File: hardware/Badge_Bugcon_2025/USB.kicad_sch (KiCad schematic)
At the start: 37 parts, among them J10 Battery, J3 USB_A, J4 USB_A, J6 USB_A, P4 USB_C_Plug_USB2.0, Q1 DMG3415U-7, SW1 ON, SW4 On, U1 USB3740B-AI9, U3 SL2.1A, U5 MCP73831T-2ATI/OT, Y5 12MHz

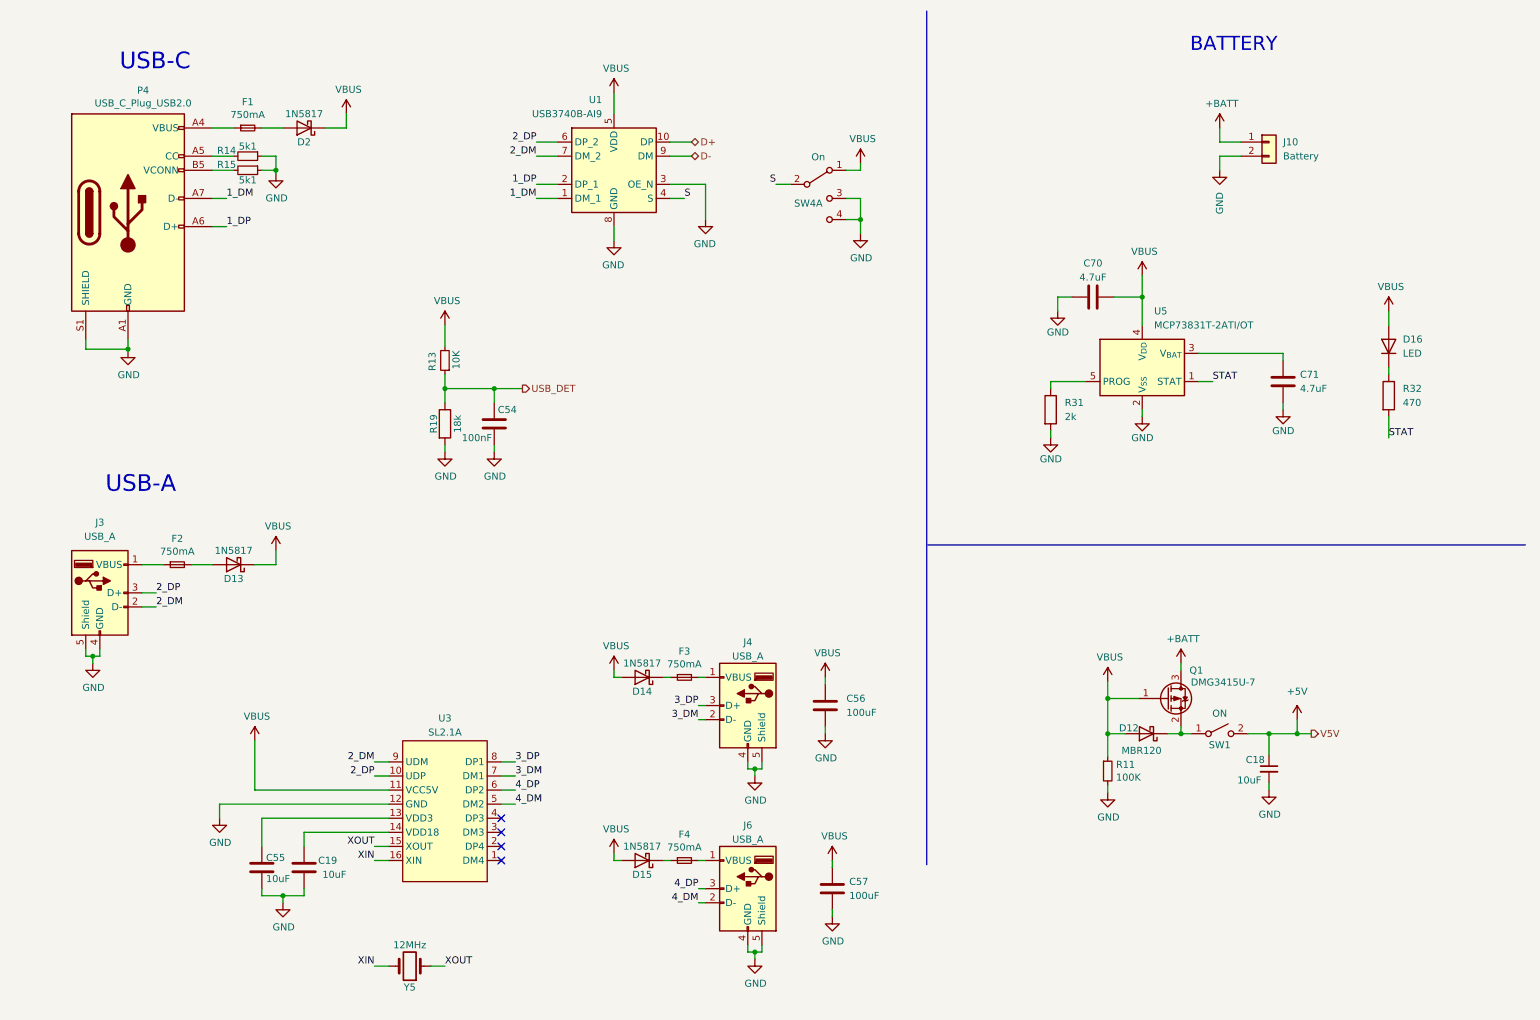
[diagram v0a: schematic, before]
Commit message: feat(Hw):Update_Schematic
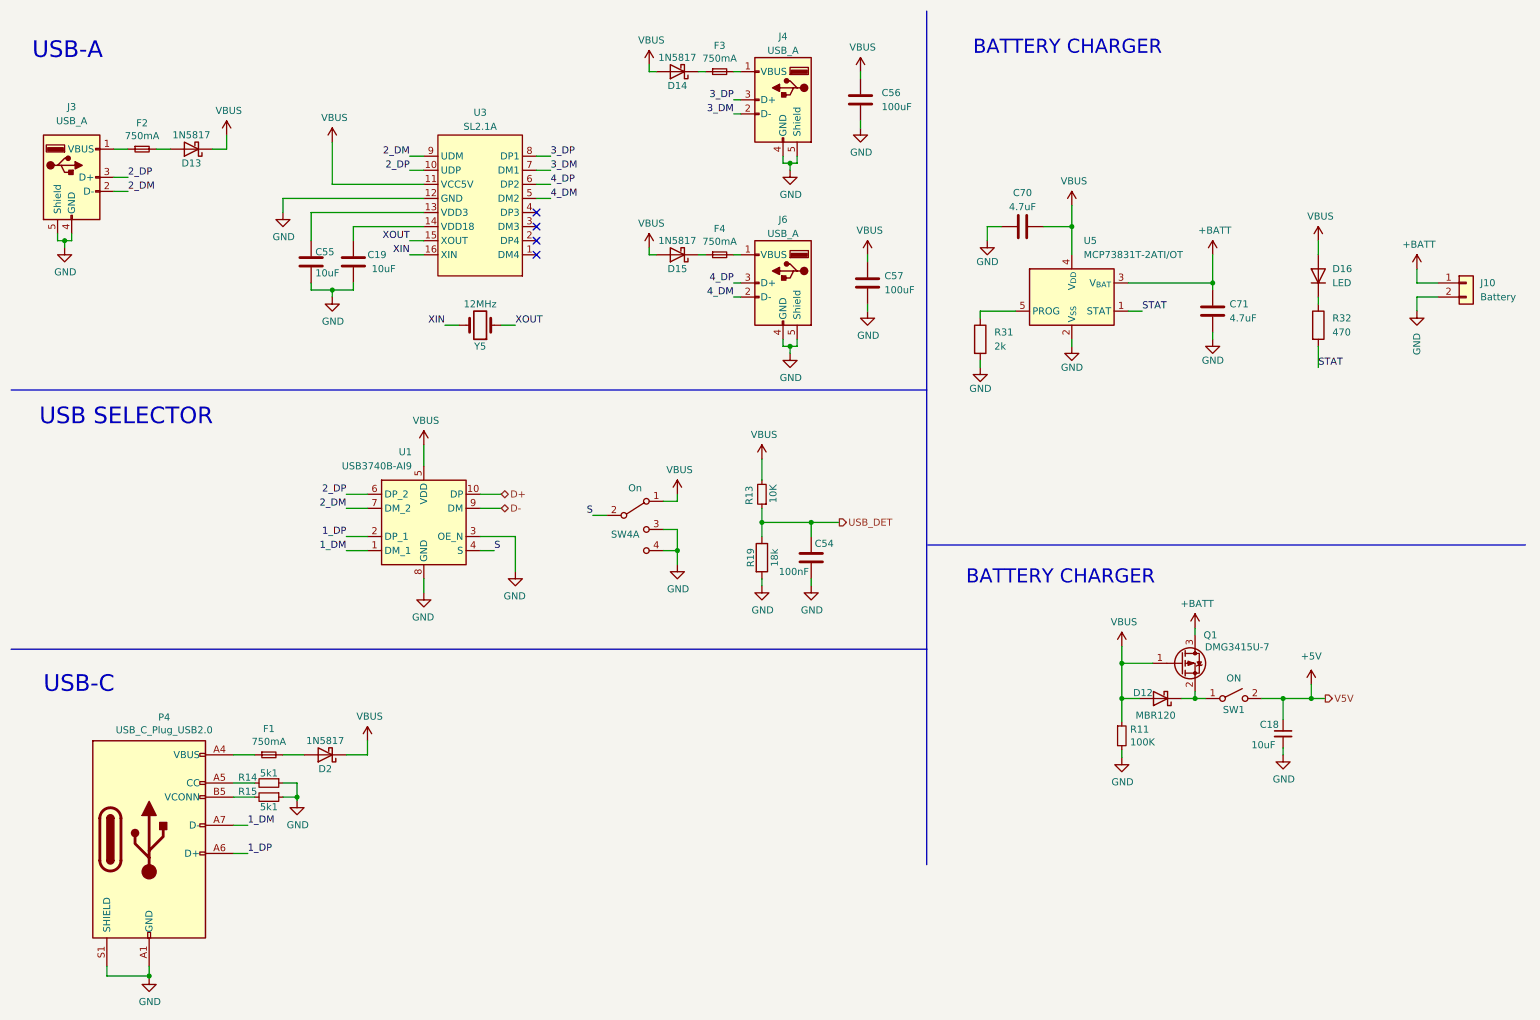
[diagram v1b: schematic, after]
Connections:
- net +BATT: now also C71.1, U5.3 (V_{BAT})
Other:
- note added: "BATTERY CHARGER"
- note added: "USB SELECTOR"
- note removed: "BATTERY"
- moved on the sheet: C18, C19, C54, C55, C56, C57, C70, C71, D12, D13, D14, D15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
